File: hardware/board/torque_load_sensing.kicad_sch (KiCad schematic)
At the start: 33 parts

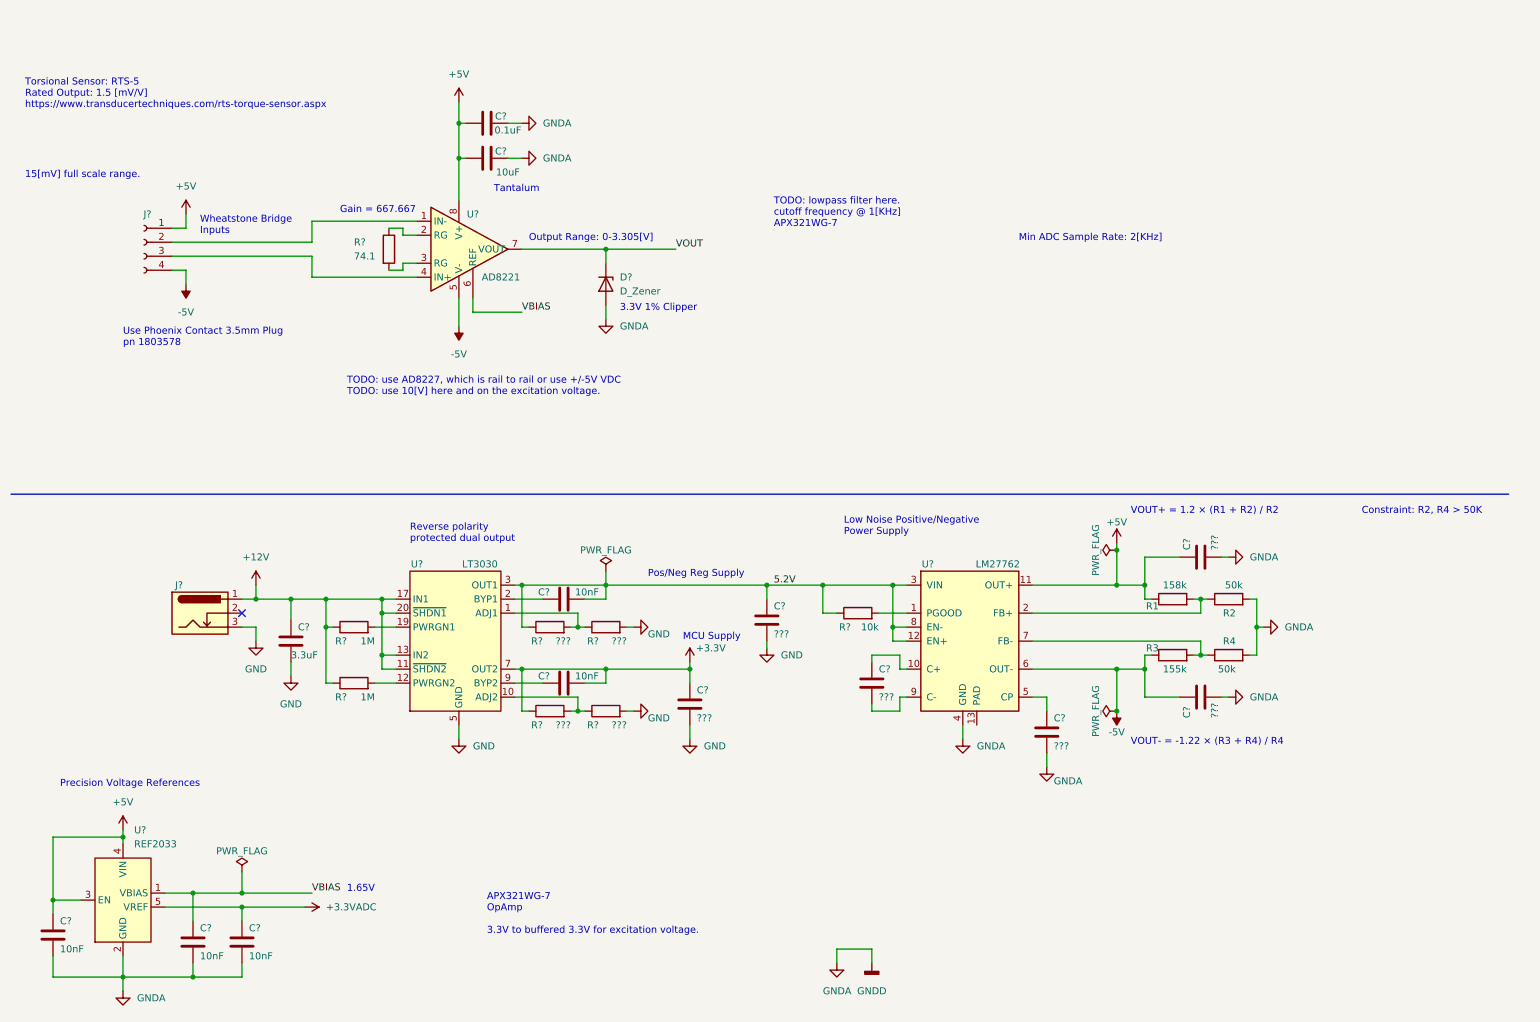
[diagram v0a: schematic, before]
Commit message: update board schematic
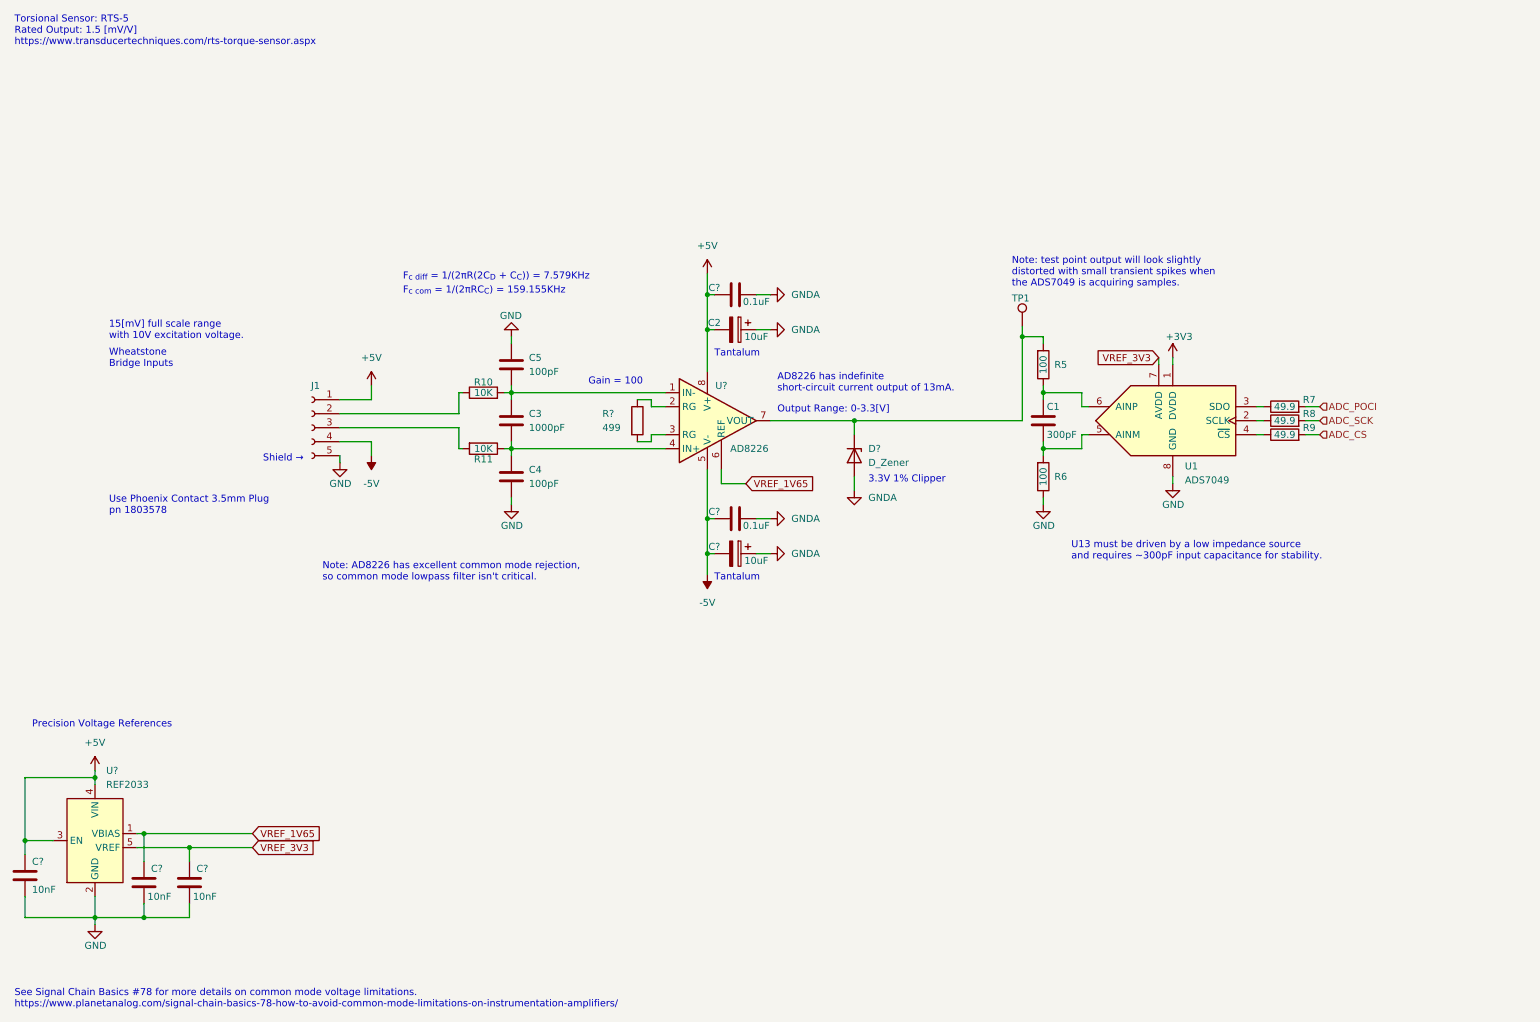
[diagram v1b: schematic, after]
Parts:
- removed C? (x6): ???, symbol Device:C
- removed C? (x2): 10nF, symbol Device:C
- removed C?: 10uF, symbol Device:C
- removed C?: 3.3uF, symbol Device:C
- removed J?: Barrel_Jack_Switch_Pin3Ring, symbol Connector:Barrel_Jack_Switch_Pin3Ring
- removed J?: Conn_01x04_Female, symbol Connector:Conn_01x04_Female
- removed R1: 158k, symbol Device:R
- removed R2, R4: 50k, symbol Device:R
- removed R3: 155k, symbol Device:R
- removed R? (x4): ???, symbol Device:R
- removed R?: 10k, symbol Device:R
- removed R? (x2): 1M, symbol Device:R
- removed U?: LT3030, symbol machine_agency_components:LT3030
- removed U?: LM27762, Package_SON:WSON-12-1EP_3x2mm_P0.5mm_EP1x2.65_ThermalVias, symbol Regulator_SwitchedCapacitor:LM27762
- added C1: 300pF, Capacitor_SMD:C_0402_1005Metric, symbol Device:C
- added C2, C?: 10uF, Capacitor_SMD:C_0805_2012Metric, symbol Device:C_Polarized
- added C3: 1000pF, symbol Device:C
- added C4, C5: 100pF, symbol Device:C
- added C?: 0.1uF, symbol Device:C
- added J1: Conn_01x05_Female, symbol Connector:Conn_01x05_Female
- added R10, R11: 10K, symbol Device:R
- added R5, R6: 100, Resistor_SMD:R_0402_1005Metric, symbol Device:R
- added R7, R8, R9: 49.9, Resistor_SMD:R_0402_1005Metric, symbol Device:R
- added TP1: TestPoint, kicad_component_library:TestPoint_Keystone_5027_Miniature, symbol Connector:TestPoint
- added U1: ADS7049, Package_SO:VSSOP-8_2.3x2mm_P0.5mm, symbol Analog_ADC:ADS7049
- R?: value 74.1 -> 499
- U?: value AD8221 -> AD8226; Link (none) -> https://www.digikey.com/en/products/detail/analog-devices-i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; Manufacturer (none) -> Analog Devices Inc.; Manufacturer Number (none) -> AD8226BRMZ-R7
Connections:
- net +3V3: now also U1.1 (DVDD)
- net +5V: now also C2.2, J1.1 (Pin_1)
- net -5V: now also C?.1, C?.2, J1.4 (Pin_4)
- net GND: now also C?.2, C?.2, C?.2, U?.2 (GND), C4.2, C5.1, J1.5 (Pin_5), R6.1, U1.8 (GND)
- net GNDA: now also C2.1, C?.1, C?.2; no longer C?.2, C?.2, C?.2, U?.2 (GND)
- net at U?.1 (IN-): now also C3.1, C5.2, R10.2
- net at U?.4 (IN+): now also C3.2, C4.1, R11.1
- net +3.3VADC renamed VREF_3V3
- net VREF_3V3: now also U1.7 (AVDD)
- net VBIAS renamed VREF_1V65
- net VOUT: no longer names the net of D?.1 (K), U?.7 (VOUT)
- net VOUT: now also R5.2, TP1.1
- new net: C1.1, R5.1, U1.6 (AINP)
- new net: R9.1, U1.4 (~{CS})
- new net: R8.1, U1.2 (SCLK)
- new net: C1.2, R6.2, U1.5 (AINM)
- new net: J1.2 (Pin_2), R10.1
- new net: J1.3 (Pin_3), R11.2
- new net: R7.1, U1.3 (SDO)
- new net ADC_CS: R9.2
- new net ADC_POCI: R7.2
- new net ADC_SCK: R8.2
- no-connect marks 1 -> 0
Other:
- note added: "15[mV] full scale range with 10V excitation voltage."
- note added: "AD8226 has indefinite short-circuit current output of 13mA."
- note added: "F_{c com} = 1/(2πRC_{C}) = 159.155KHz"
- note added: "F_{c diff} = 1/(2πR(2C_{D} + C_{C})) = 7.579KHz"
- note added: "Gain = 100"
- note added: "Note: AD8226 has excellent common mode rejection, so common mode lowpass filter isn't critical."
- note added: "Note: test point output will look slightly distorted with small transient spikes when the ADS7049 is acquiring samples."
- note added: "Output Range: 0-3.3[V]"
- note added: "See Signal Chain Basics #78 for more details on common mode voltage limitations. https://www.planetanalog.com/signal-chain-basics-78-how-to-avoid-common-mode-limitations-on-instrumentation-amplifiers/"
- note added: "Shield →"
- note added: "U13 must be driven by a low impedance source and requires ~300pF input capacitance for stability."
- note removed: "1.65V"
- note removed: "15[mV] full scale range."
- note removed: "APX321WG-7 OpAmp 3.3V to buffered 3.3V for excitation voltage."
- note removed: "Constraint: R2, R4 > 50K"
- note removed: "Gain = 667.667"
- note removed: "Low Noise Positive/Negative Power Supply"
- note removed: "MCU Supply"
- note removed: "Min ADC Sample Rate: 2[KHz]"
- note removed: "Output Range: 0-3.305[V]"
- note removed: "Pos/Neg Reg Supply"
- note removed: "Reverse polarity protected dual output"
- note removed: "TODO: lowpass filter here. cutoff frequency @ 1[KHz] APX321WG-7"
- note removed: "TODO: use AD8227, which is rail to rail or use +/-5V VDC TODO: use 10[V] here and on the excitation voltage."
- note removed: "VOUT+ = 1.2 × (R1 + R2) / R2"
- note removed: "VOUT- = -1.22 × (R3 + R4) / R4"
- moved on the sheet: C?, D?, R?, U?
